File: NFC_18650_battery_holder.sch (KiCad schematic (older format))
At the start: 2 parts

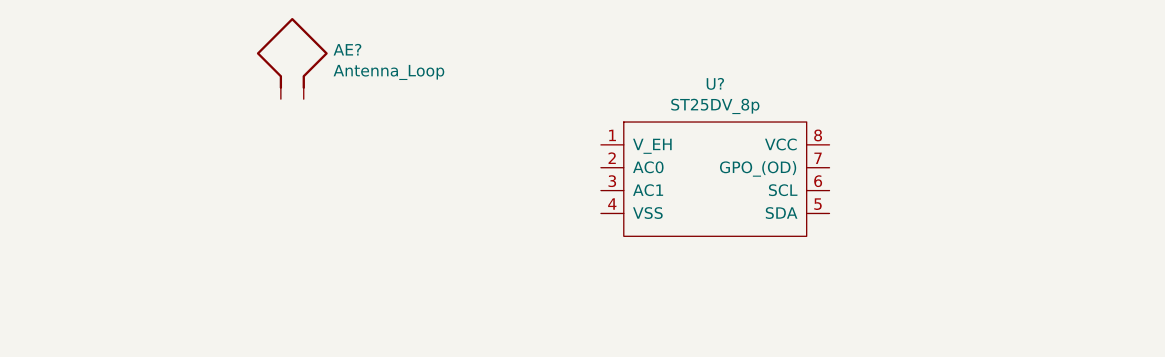
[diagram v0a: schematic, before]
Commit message: Schematic done.
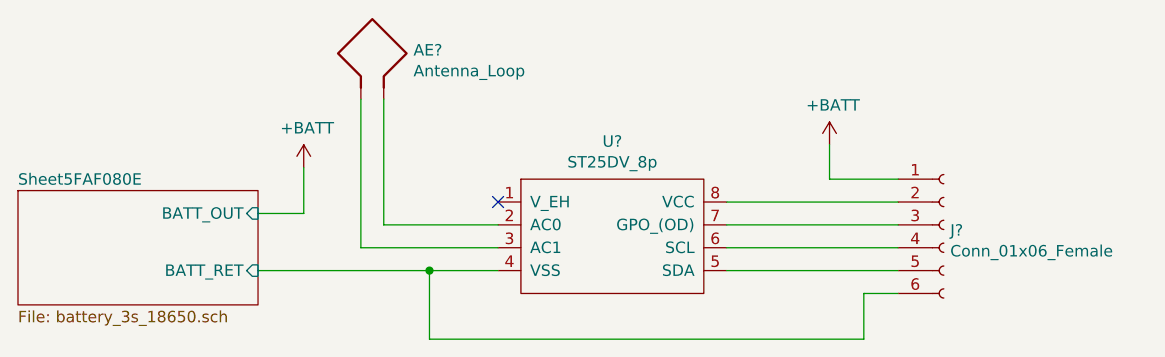
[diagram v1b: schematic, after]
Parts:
- added J?: Conn_01x06_Female, symbol Connector:Conn_01x06_Female
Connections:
- net at AE?.1: now also U?.3 (AC1)
- net at AE?.2: now also U?.2 (AC0)
- net Sheet5FAF080E/BATT_RET: now reaches U?.4 (VSS)
- net Sheet5FAF080E/BATT_RET: now also J?.6 (Pin_6)
- net at U?.5 (SDA): now also J?.5 (Pin_5)
- net at U?.6 (SCL): now also J?.4 (Pin_4)
- net at U?.7 (GPO_(OD)): now also J?.3 (Pin_3)
- net at U?.8 (VCC): now also J?.2 (Pin_2)
- new net +BATT: J?.1 (Pin_1)
- no-connect marks 0 -> 1
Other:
- moved on the sheet: AE?, U?
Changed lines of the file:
@@
 $Descr A4 11693 8268
 encoding utf-8
-Sheet 1 1
+Sheet 1 2
 Title ""
 Date ""
@@
 L Device:Antenna_Loop AE?
 U 1 1 5FAE3919
-P 6700 2400
-F 0 "AE?" H 6930 2414 50  0000 L CNN
-F 1 "Antenna_Loop" H 6930 2323 50  0000 L CNN
-F 2 "" H 6700 2400 50  0001 C CNN
-F 3 "~" H 6700 2400 50  0001 C CNN
-	1    6700 2400
+P 7050 2400
+F 0 "AE?" H 7280 2414 50  0000 L CNN
+F 1 "Antenna_Loop" H 7280 2323 50  0000 L CNN
+F 2 "" H 7050 2400 50  0001 C CNN
+F 3 "~" H 7050 2400 50  0001 C CNN
+	1    7050 2400
 	1    0    0    -1
 $EndComp
@@
 L NFC_18659_battery_holder:ST25DV_8p U?
 U 1 1 5FAE5573
-P 8600 2550
-F 0 "U?" H 8600 2565 50  0000 C CNN
-F 1 "ST25DV_8p" H 8600 2474 50  0000 C CNN
-F 2 "" H 8600 2550 50  0001 C CNN
-F 3 "" H 8600 2550 50  0001 C CNN
-	1    8600 2550
+P 8150 2800
+F 0 "U?" H 8150 2815 50  0000 C CNN
+F 1 "ST25DV_8p" H 8150 2724 50  0000 C CNN
+F 2 "" H 8150 2800 50  0001 C CNN
+F 3 "" H 8150 2800 50  0001 C CNN
+	1    8150 2800
 	1    0    0    -1
 $EndComp
+$Sheet
+S 5550 3000 1050 500
+U 5FAF080F
+F0 "Sheet5FAF080E" 50
+F1 "battery_3s_18650.sch" 50
+F2 "BATT_OUT" I R 6600 3100 50
+F3 "BATT_RET" I R 6600 3350 50
+$EndSheet
+Wire Wire Line
+	7650 3150 7150 3150
+Wire Wire Line
+	7150 3150 7150 2600
+Wire Wire Line
+	7050 2600 7050 3250
+Wire Wire Line
+	7050 3250 7650 3250
+Wire Wire Line
+	7650 3350 7350 3350
+$Comp
+L power:+BATT #PWR?
+U 1 1 5FAF9693
+P 6800 2900
+F 0 "#PWR?" H 6800 2750 50  0001 C CNN
+F 1 "+BATT" H 6815 3073 50  0000 C CNN
+F 2 "" H 6800 2900 50  0001 C CNN
+F 3 "" H 6800 2900 50  0001 C CNN
+	1    6800 2900
+	1    0    0    -1
+$EndComp
+Wire Wire Line
+	6800 3100 6800 2900
+Wire Wire Line
+	6600 3100 6800 3100
+Wire Wire Line
+	9400 3350 8650 3350
+Wire Wire Line
+	8650 3250 9400 3250
+Wire Wire Line
+	9400 3150 8650 3150
+Wire Wire Line
+	8650 3050 9400 3050
+Wire Wire Line
+	9400 2950 9100 2950
+Wire Wire Line
+	9100 2950 9100 2800
+$Comp
+L power:+BATT #PWR?
+U 1 1 5FAFB912
+P 9100 2800
+F 0 "#PWR?" H 9100 2650 50  0001 C CNN
+F 1 "+BATT" H 9115 2973 50  0000 C CNN
+F 2 "" H 9100 2800 50  0001 C CNN
+F 3 "" H 9100 2800 50  0001 C CNN
+	1    9100 2800
+	1    0    0    -1
+$EndComp
+$Comp
+L Connector:Conn_01x06_Female J?
+U 1 1 5FAFC15A
+P 9600 3150
+F 0 "J?" H 9628 3126 50  0000 L CNN
+F 1 "Conn_01x06_Female" H 9628 3035 50  0000 L CNN
+F 2 "" H 9600 3150 50  0001 C CNN
+F 3 "~" H 9600 3150 50  0001 C CNN
+	1    9600 3150
+	1    0    0    -1
+$EndComp
+Wire Wire Line
+	9400 3450 9250 3450
+Wire Wire Line
+	9250 3450 9250 3650
+Wire Wire Line
+	9250 3650 7350 3650
+Wire Wire Line
+	7350 3650 7350 3350
+Connection ~ 7350 3350
+Wire Wire Line
+	7350 3350 6600 3350
+NoConn ~ 7650 3050
 $EndSCHEMATC
